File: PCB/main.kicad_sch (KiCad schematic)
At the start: 8 parts, among them U1 MCP2558FD, U2 MCP2558FD, U3 STM32G0B1, Y1 ${Frequency}

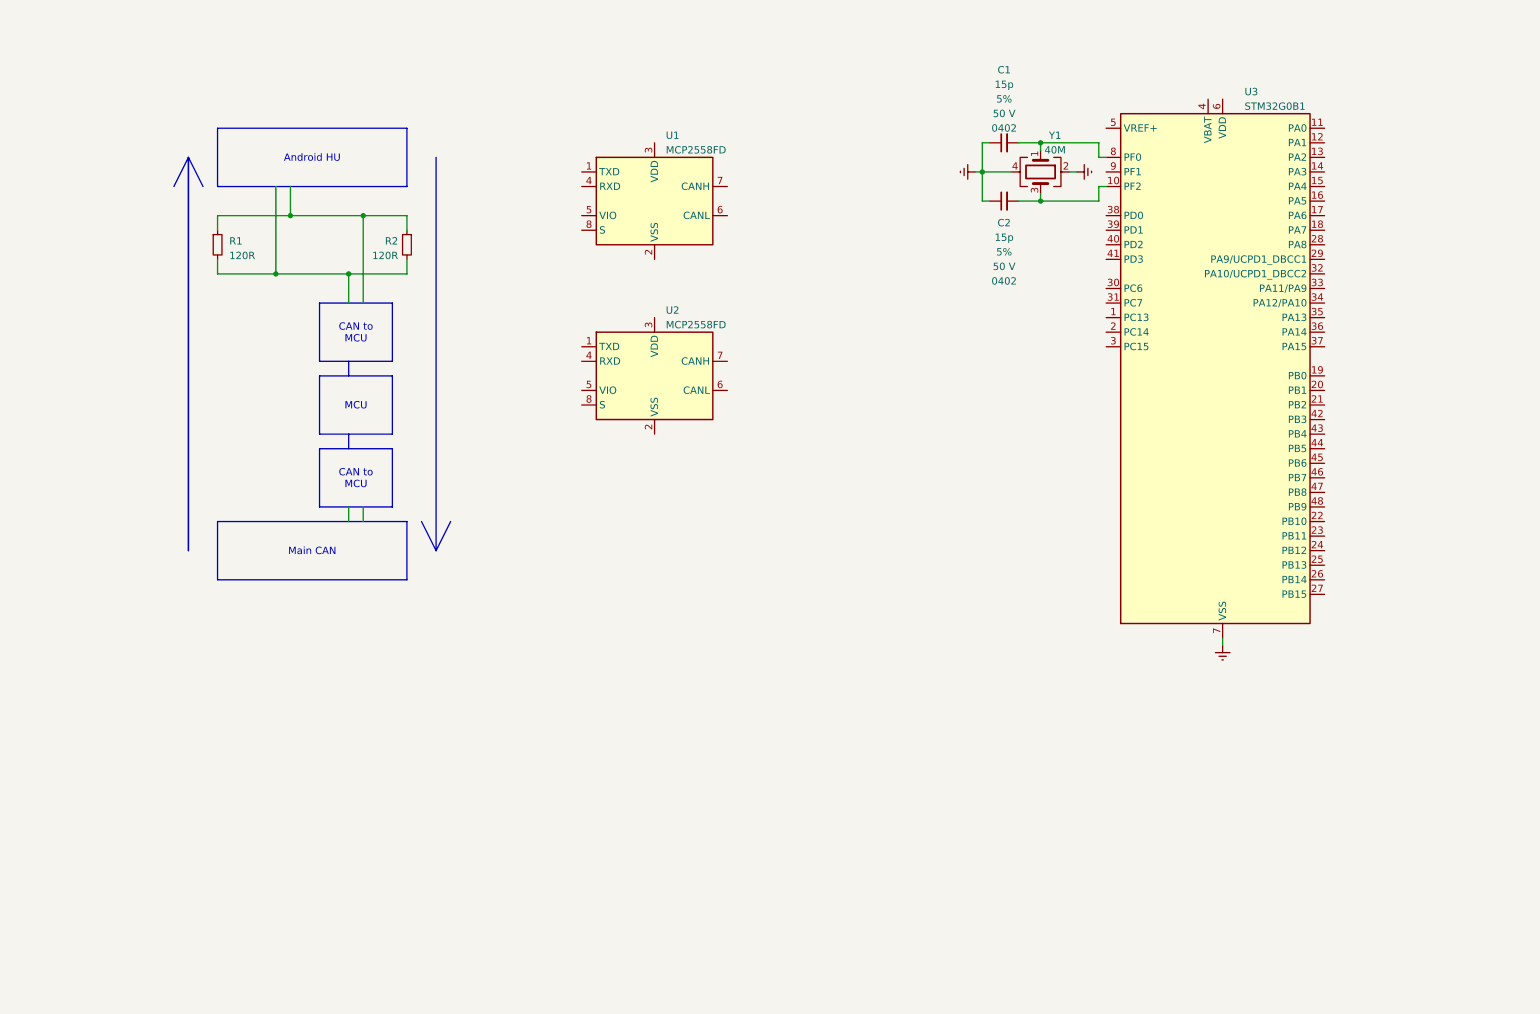
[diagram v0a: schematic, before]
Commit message: Develop board
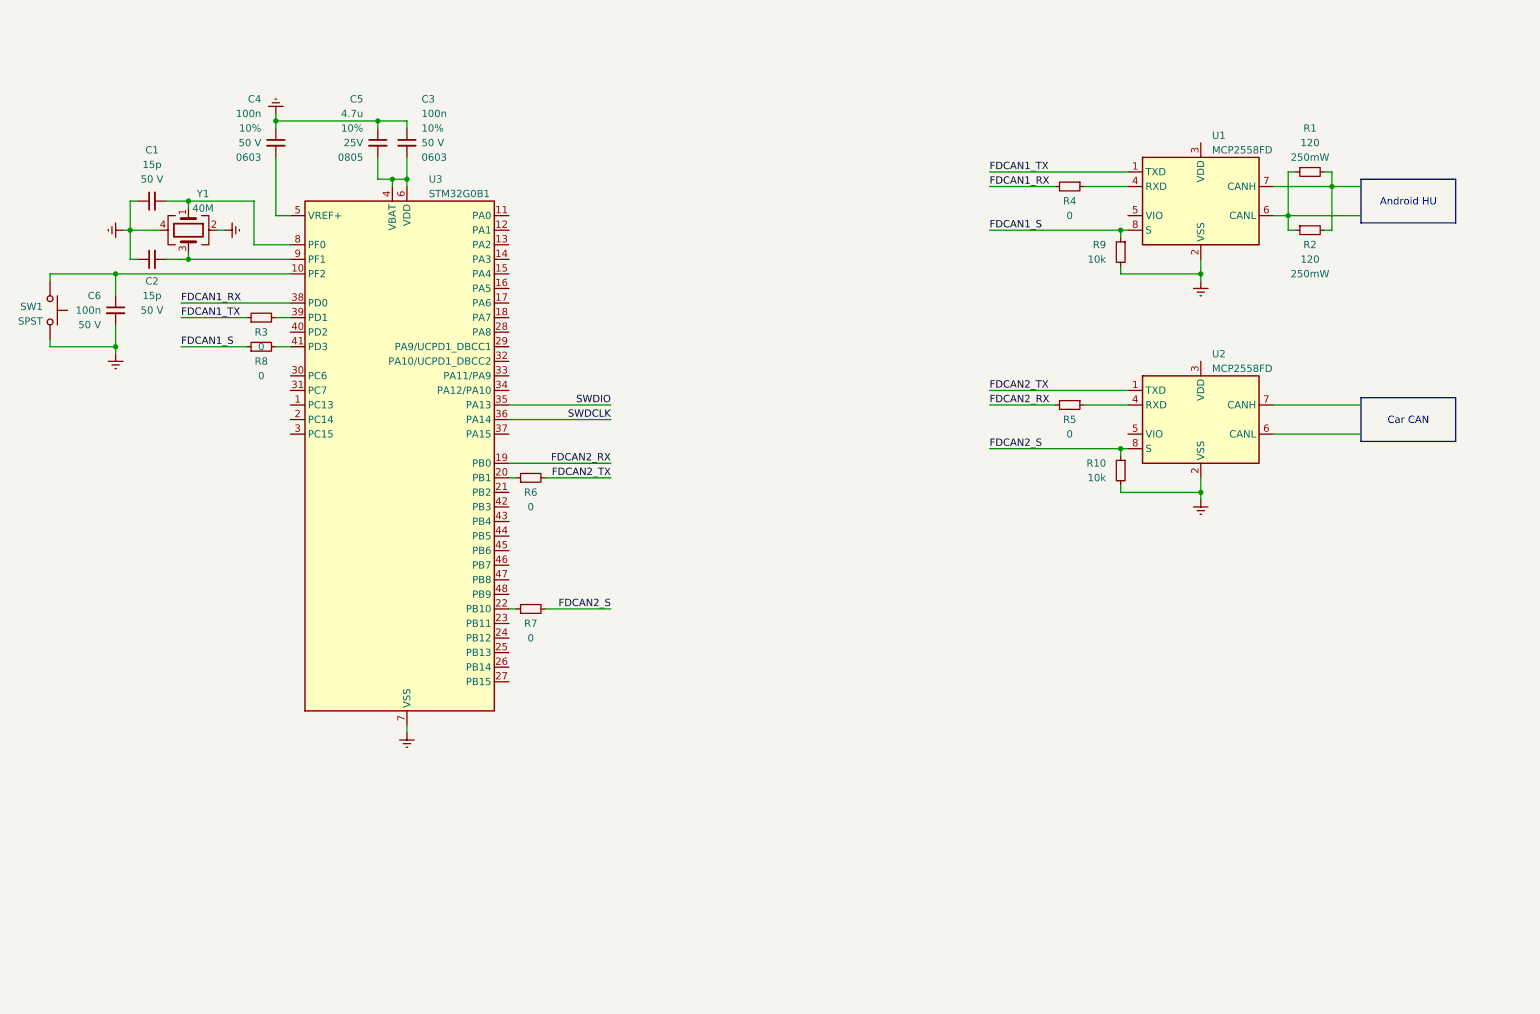
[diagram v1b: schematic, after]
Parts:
- removed R1, R2: 120R, symbol Device:R_Small
- added C3, C4, C6: ${Capacitance}, Capacitor_SMD:C_0603_1608Metric, symbol 0 LibDB:Capacitors/CMP-0008
- added C5: ${Capacitance}, Capacitor_SMD:C_0805_2012Metric, symbol 0 LibDB:Capacitors/CMP-0009
- added R1, R2: ${Resistance}, Resistor_SMD:R_1206_3216Metric, symbol 0 LibDB:Resistors/CMP-0006
- added R10, R9: ${Resistance}, Resistor_SMD:R_0402_1005Metric, symbol 0 LibDB:Resistors/CMP-0010
- added R3, R4, R5, R6, R7, R8: ${Resistance}, Resistor_SMD:R_0402_1005Metric, symbol 0 LibDB:Resistors/CMP-0007
- added SW1: SPST, libdb:CMP-0011, symbol 0 LibDB:Switches/CMP-0011
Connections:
- net Earth: now also U1.2 (VSS), U2.2 (VSS), C3.1, C4.1, C5.1, C6.2, R10.2, R9.2, SW1.1
- net FDCAN1_TX: now reaches U1.1 (TXD)
- net FDCAN1_TX: now also R3.1
- net at U1.4 (RXD): now also R4.1
- net at U1.6 (CANL): now also R1.1, R2.1
- net at U1.7 (CANH): now also R1.2, R2.2
- net FDCAN1_S: now reaches U1.8 (S)
- net FDCAN1_S: now also R8.1, R9.1
- net at C2.2, Y1.3: now also U3.9 (PF1); no longer U3.10 (PF2)
- net FDCAN2_TX: now reaches U2.1 (TXD)
- net FDCAN2_TX: now also R6.2
- net at U2.4 (RXD): now also R5.1
- net FDCAN2_S: now reaches U2.8 (S)
- net FDCAN2_S: now also R10.1, R7.2
- net FDCAN2_RX: now reaches U3.19 (PB0)
- net FDCAN2_RX: now also R5.2
- net at U3.20 (PB1): now also R6.1
- net at U3.22 (PB10): now also R7.1
- net SWDIO: now reaches U3.35 (PA13)
- net SWDCLK: now reaches U3.36 (PA14)
- net FDCAN1_RX: now reaches U3.38 (PD0)
- net FDCAN1_RX: now also R4.2
- net at U3.39 (PD1): now also R3.2
- net at U3.4 (VBAT): now also U3.6 (VDD), C3.2, C5.2
- net at U3.41 (PD3): now also R8.2
- net at U3.5 (VREF+): now also C4.2
- new net: C6.1, SW1.2, U3.10 (PF2)
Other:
- moved on the sheet: C1, C2, U1, U2, U3, Y1

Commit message: Further develop board
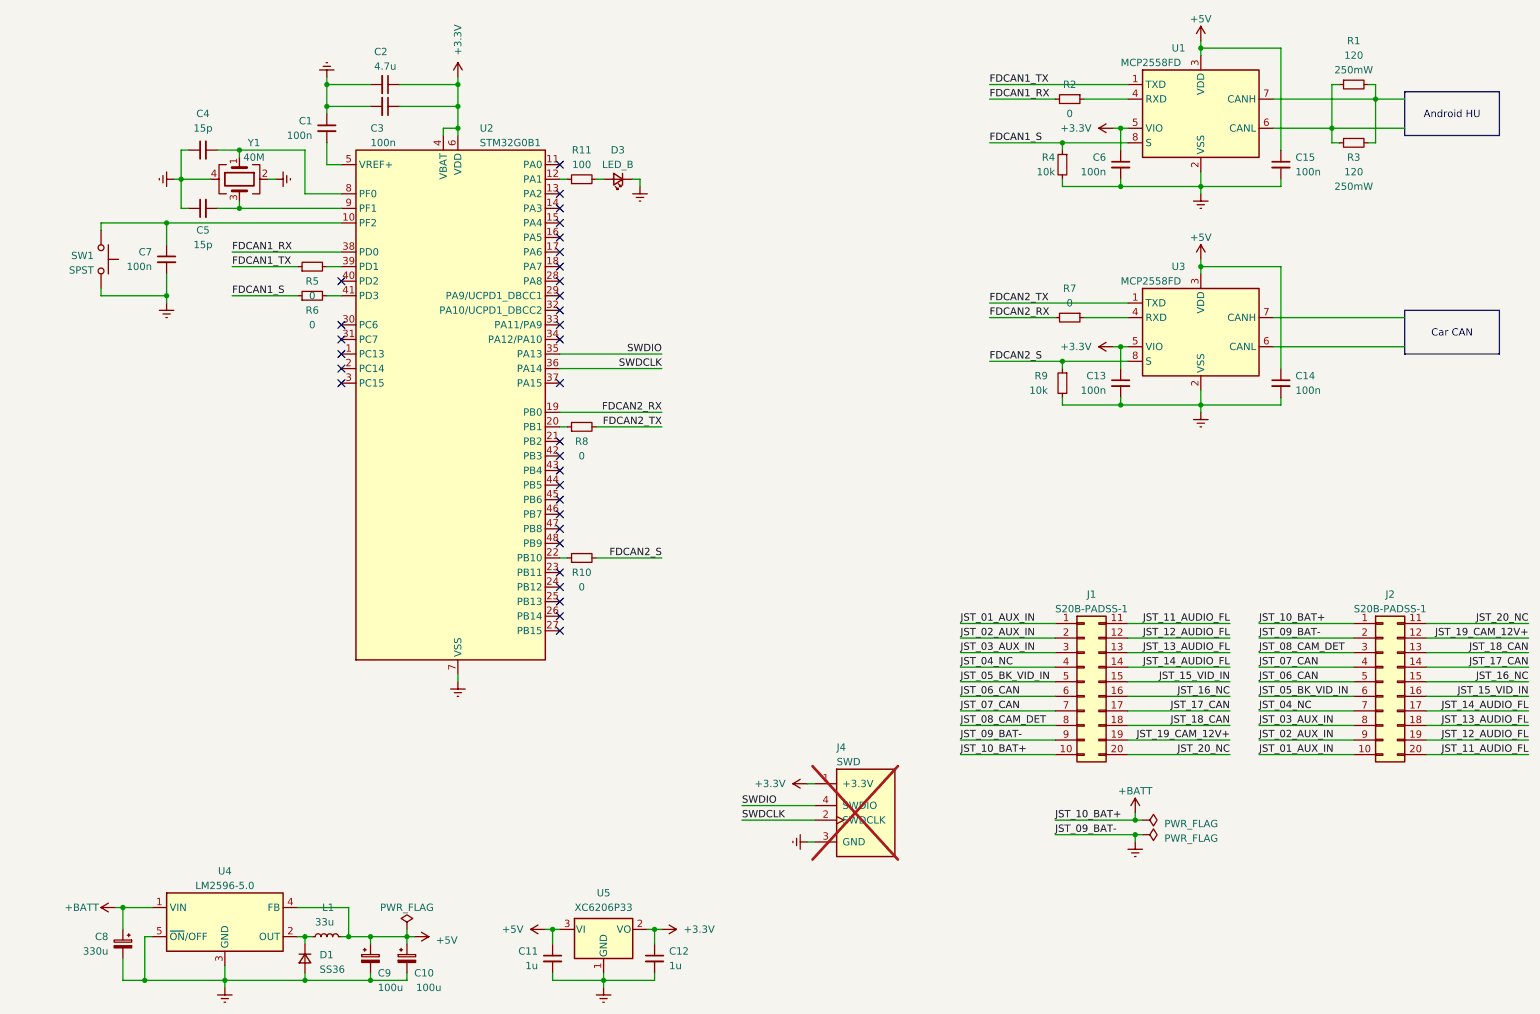
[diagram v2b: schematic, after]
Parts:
- added C10, C9: ${Capacitance}, Capacitor_Tantalum_SMD:CP_EIA-3528-15_AVX-H, symbol 0 LibDB:Capacitors/CMP-0017
- added C11, C12: ${Capacitance}, Capacitor_SMD:C_0805_2012Metric, symbol 0 LibDB:Capacitors/CMP-0020
- added C13, C14, C15, C6: ${Capacitance}, Capacitor_SMD:C_0402_1005Metric, symbol 0 LibDB:Capacitors/CMP-0021
- added C8: ${Capacitance}, Capacitor_SMD:CP_Elec_10x10, symbol 0 LibDB:Capacitors/CMP-0018
- added D1: SS36, Diode_SMD:D_SMC, symbol 0 LibDB:Schottky Diodes/CMP-0016
- added D3: LED_B, Device:LED_Small, symbol 0 LibDB:LEDs/CMP-0023
- added J1, J2: S20B-PADSS-1, libdb:CMP-0012, symbol 0 LibDB:Connectors/CMP-0012
- added J4: SWD, libdb:CMP-0022, symbol 0 LibDB:Connectors/CMP-0022
- added L1: ${Inductance}, Inductor_SMD:L_1210_3225Metric, symbol 0 LibDB:Inductors/CMP-0015
- added R11: ${Resistance}, Resistor_SMD:R_0402_1005Metric, symbol 0 LibDB:Resistors/CMP-0024
- added U4: LM2596-5.0, Package_TO_SOT_SMD:TO-263-5_TabPin3, symbol 0 LibDB:DC-DC Converters/CMP-0014
- added U5: XC6206P33, libdb:CMP-0019, symbol 0 LibDB:LDO Regulators/CMP-0019
- C1: renamed from C4; Voltage Rating 50 V -> 50V
- C3: Voltage Rating 50 V -> 50V
- C4: renamed from C1; Voltage Rating 50 V -> 50V
- C5: renamed from C2; Voltage Rating 50 V -> 50V
- C7: renamed from C6; Voltage Rating 50 V -> 50V
- U1: Manufacturer Microchip Technology -> Microchip Technology
- U3: renamed from U2; Manufacturer Microchip Technology -> Microchip Technology
- Y1: footprint Crystal:Crystal_SMD_2016-4Pin_2.0x1.6mm -> libdb:CMP-0004
- renumbered C5 to C2, R7 to R10, R4 to R2, R2 to R3, R9 to R4, R3 to R5, R8 to R6, R5 to R7, R6 to R8, R10 to R9, U3 to U2
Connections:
- net Earth: now also C2.2, C3.2, C10.2, C11.2, C12.2, C13.2, C14.2, C15.2, C6.2, C8.2, C9.2, D1.2 (A), D3.1 (K), J1.9 (Pin_9), J2.2 (Pin_2), J4.3 (GND), U4.3 (GND), U4.5 (~{ON}/OFF), U5.1 (GND); no longer C2.1, C3.1
- net SWDCLK: now also J4.2 (SWDCLK)
- net SWDIO: now also J4.4 (SWDIO)
- net +5V: now reaches U1.3 (VDD)
- net +5V: now also U3.3 (VDD), C10.1, C11.1, C14.1, C15.1, C9.1, L1.2, U4.4 (FB), U5.3 (VI)
- net +3.3V: now reaches U1.5 (VIO)
- net +3.3V: now also C2.1, C3.1, U2.4 (VBAT), U2.6 (VDD), U3.5 (VIO), C12.1, C13.1, C6.1, J4.1 (+3.3V), U5.2 (VO)
- net at U2.12 (PA1): now also R11.1
- new net: D1.1 (K), L1.1, U4.2 (OUT)
- new net: D3.2 (A), R11.2
- new net +BATT: C8.1, J1.10 (Pin_10), J2.1 (Pin_1), U4.1 (VIN)
- new net JST_01_AUX_IN: J1.1 (Pin_1), J2.10 (Pin_10)
- new net JST_02_AUX_IN: J1.2 (Pin_2), J2.9 (Pin_9)
- new net JST_03_AUX_IN: J1.3 (Pin_3), J2.8 (Pin_8)
- new net JST_04_NC: J1.4 (Pin_4), J2.7 (Pin_7)
- new net JST_05_BK_VID_IN: J1.5 (Pin_5), J2.6 (Pin_6)
- new net JST_06_CAN: J1.6 (Pin_6), J2.5 (Pin_5)
- new net JST_07_CAN: J1.7 (Pin_7), J2.4 (Pin_4)
- new net JST_08_CAM_DET: J1.8 (Pin_8), J2.3 (Pin_3)
- new net JST_11_AUDIO_FL: J1.11 (Pin_11), J2.20 (Pin_20)
- new net JST_12_AUDIO_FL: J1.12 (Pin_12), J2.19 (Pin_19)
- new net JST_13_AUDIO_FL: J1.13 (Pin_13), J2.18 (Pin_18)
- new net JST_14_AUDIO_FL: J1.14 (Pin_14), J2.17 (Pin_17)
- new net JST_15_VID_IN: J1.15 (Pin_15), J2.16 (Pin_16)
- new net JST_16_NC: J1.16 (Pin_16), J2.15 (Pin_15)
- new net JST_17_CAN: J1.17 (Pin_17), J2.14 (Pin_14)
- new net JST_18_CAN: J1.18 (Pin_18), J2.13 (Pin_13)
- new net JST_19_CAM_12V+: J1.19 (Pin_19), J2.12 (Pin_12)
- new net JST_20_NC: J1.20 (Pin_20), J2.11 (Pin_11)
- no-connect marks 0 -> 32
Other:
- moved on the sheet: C1, C2, C3, C4, C5, C7, R1, R10, R2, R3, R4, R5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
